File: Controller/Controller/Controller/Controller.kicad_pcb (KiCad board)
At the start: 4 copper layers, 121 x 80 mm, 124 parts, among them J1 Conn_01x02, J2 Conn_02x20_Counter_Clockwise, J3 Conn_01x06, J4 Conn_01x05, J5 USB_A, J6 USB_C_Receptacle_USB2.0, J7 RJ45_Amphenol_RJMG1BD3B8K1ANR, J8 Conn_01x06_MountingPin, J9 Conn_01x50_MountingPin, Q1 CSD16323Q3, SW1 SW_Push, SW2 SW_Push, U1 STM32F746IGTx, U10 LTC1261L, U2 LAN8720A, U3 M24C02-WMN, U4 LM317_TO-252, U5 AMS1117-3.3, U6 LM317_TO-252, U7 LM3488, U8 C85037, U9 LM317_TO-252, X1 XO32, Y1 32.765Mhz

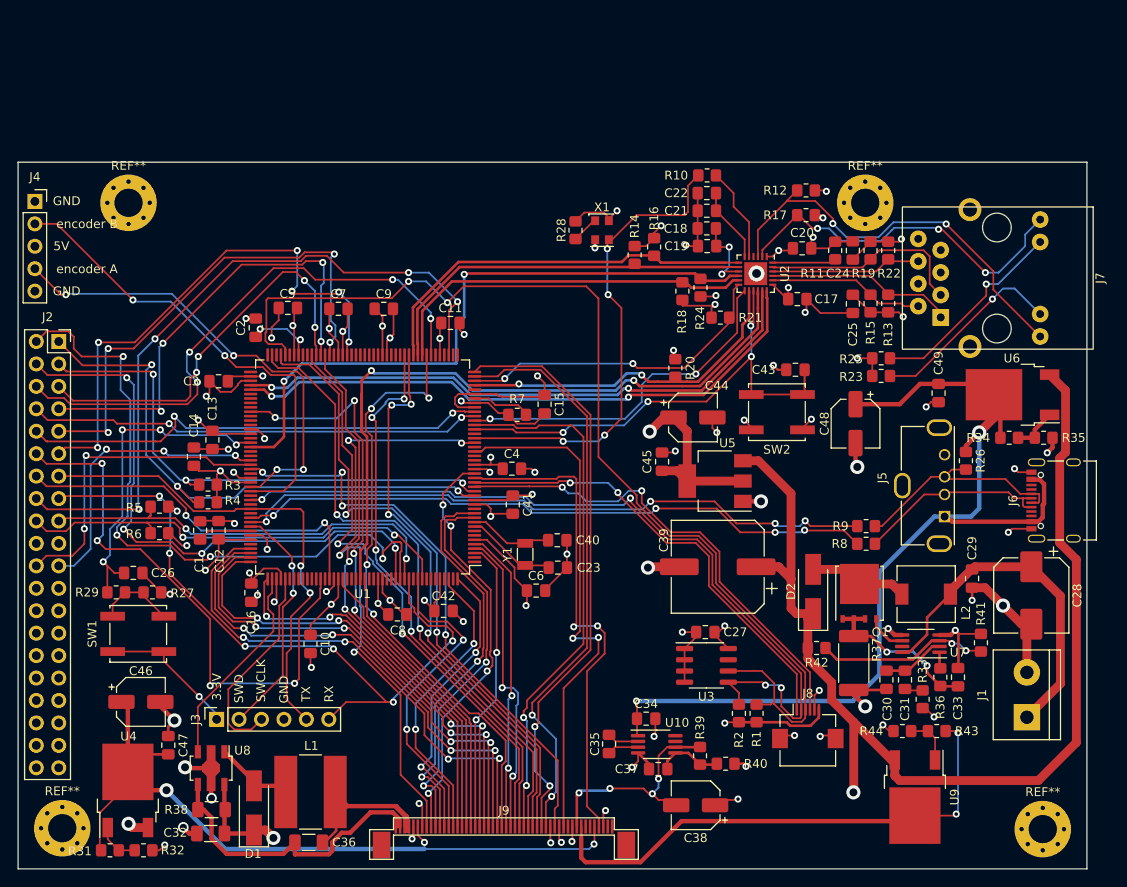
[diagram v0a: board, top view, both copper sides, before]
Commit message: contoller and contoller front Rev 1
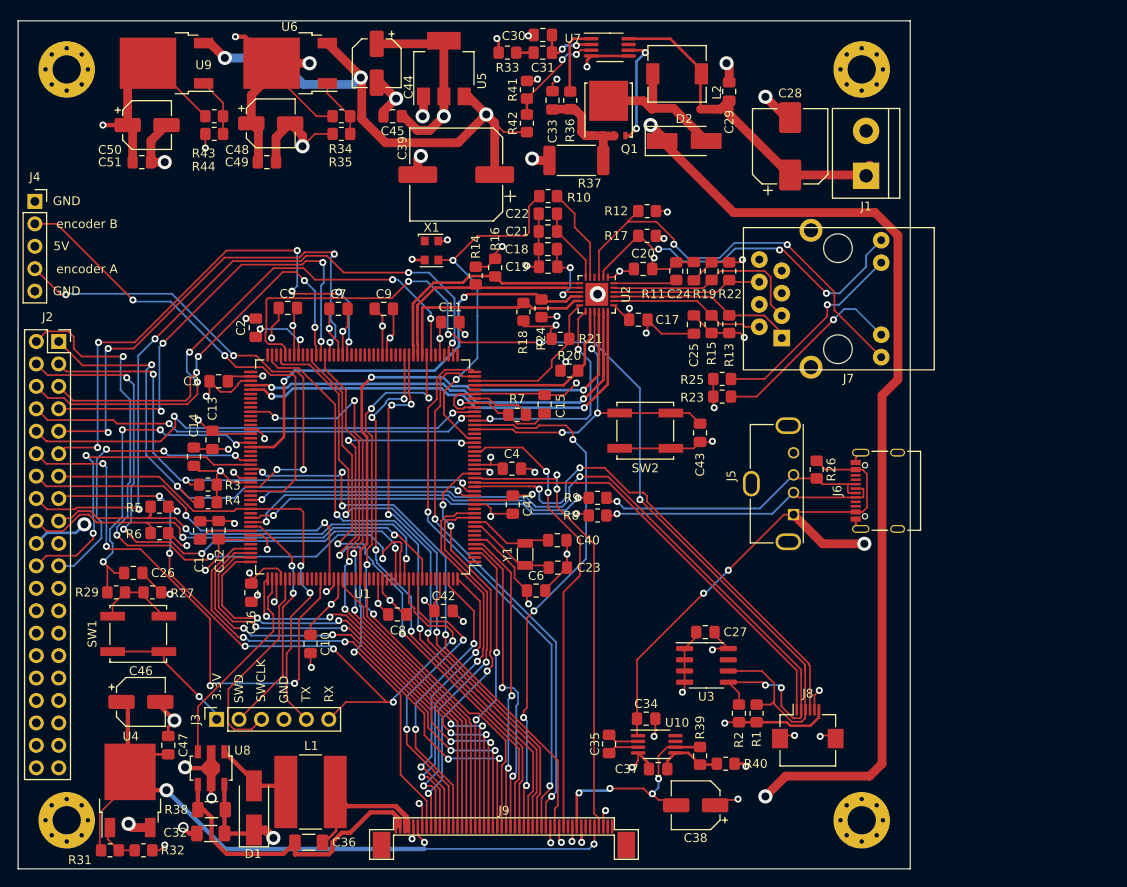
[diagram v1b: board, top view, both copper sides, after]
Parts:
- removed R28: 10Kohm, Resistor_SMD:R_0805_2012Metric_Pad1.20x1.40mm_HandSolder
- removed the REF** at (71.0, 120.4)
- removed the REF** at (182.0, 120.5)
- removed the REF** at (78.5, 49.6)
- removed the REF** at (161.9, 49.6)
- added C50: 100uF, Capacitor_SMD:CP_Elec_5x5.4, F.Cu at (80.6, 40.8)
- added C51: 4.7uF, Capacitor_SMD:C_0805_2012Metric_Pad1.18x1.45mm_HandSolder, F.Cu at (80.0, 45.0)
- added R: MountingHole_3.2mm_M3_Pad_Via, MountingHole:MountingHole_3.2mm_M3_Pad_Via, F.Cu at (71.5, 119.5)
- added REF**: MountingHole_3.2mm_M3_Pad_Via, MountingHole:MountingHole_3.2mm_M3_Pad_Via, F.Cu at (71.5, 34.5)
- added REF**: MountingHole_3.2mm_M3_Pad_Via, MountingHole:MountingHole_3.2mm_M3_Pad_Via, F.Cu at (161.5, 119.5)
- added REF**: MountingHole_3.2mm_M3_Pad_Via, MountingHole:MountingHole_3.2mm_M3_Pad_Via, F.Cu at (161.5, 34.5)
- moved U9 118.7 mm to (82.8, 33.8), turned to 180 degrees
- moved R43 107.4 mm to (88.2, 39.8), turned to 0 degrees
- moved R44 103.1 mm to (88.2, 41.8)
- moved U6 90.0 mm to (96.8, 33.8)
- moved R33 87.0 mm to (121.4, 32.6), turned to 180 degrees
- moved R35 86.6 mm to (102.6, 41.8), turned to 180 degrees
- moved R34 83.9 mm to (102.6, 39.8)
- moved C30 82.7 mm to (125.4, 30.6), turned to 180 degrees
- moved C31 82.0 mm to (125.4, 32.6), turned to 180 degrees
- moved R41 81.0 mm to (123.6, 36.8)
- moved C49 80.4 mm to (94.2, 45.0), turned to 0 degrees
- moved C33 79.8 mm to (126.5, 38.0)
- moved R36 77.6 mm to (128.5, 38.0)
- moved U7 76.1 mm to (133.0, 32.0), turned to 0 degrees
- moved C48 74.4 mm to (94.6, 40.6), turned to 0 degrees
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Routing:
- net 9.6V: track 58.3 -> 177.9 mm
- net 18V: track 236.3 -> 288.9 mm, vias 4 -> 8
- net Net-(R8-Pad1): track 72.3 -> 40.0 mm, vias 4 -> 2
- net Net-(R9-Pad1): track 73.2 -> 41.4 mm, vias 4 -> 2
- net RMII_TXEN: track 81.3 -> 58.1 mm
- net RMII_RXER: track 73.8 -> 52.1 mm
- net RMII_RXD-: track 45.7 -> 25.8 mm
- net RMII_MDIO: track 37.3 -> 17.8 mm, vias 2 -> 0
- net RMII_REF_CLK: track 39.2 -> 19.7 mm, vias 2 -> 0
- net RMII_CRS_DV: track 43.6 -> 24.5 mm
- net RMII_RXD+: track 45.0 -> 26.3 mm
- net RMII_TXD+: track 68.1 -> 51.4 mm
- net RESET: track 55.3 -> 39.3 mm, vias 4 -> 3
- net RMII_TXD-: track 67.0 -> 52.9 mm
- net RMII_MDC: track 40.1 -> 26.0 mm
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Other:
- board size 121 x 80 mm -> 101 x 96 mm
